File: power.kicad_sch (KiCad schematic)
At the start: 18 parts, among them U3 RT8096B

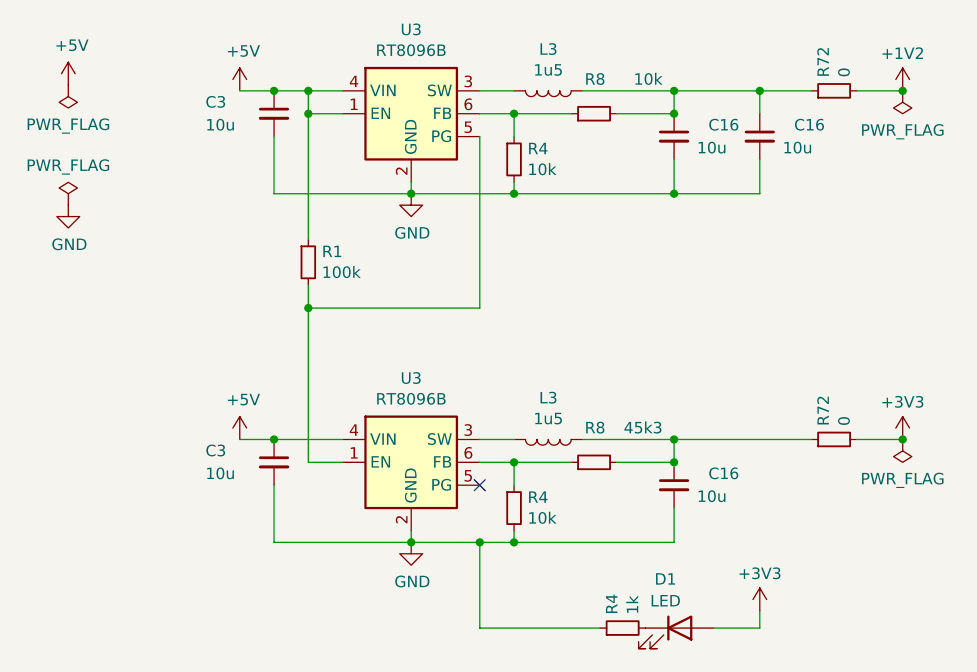
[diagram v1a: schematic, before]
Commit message: sdram layout done - COMPLETE REWORK NEEDED
cannot mix LVDS and GPIO banks due to too different timing
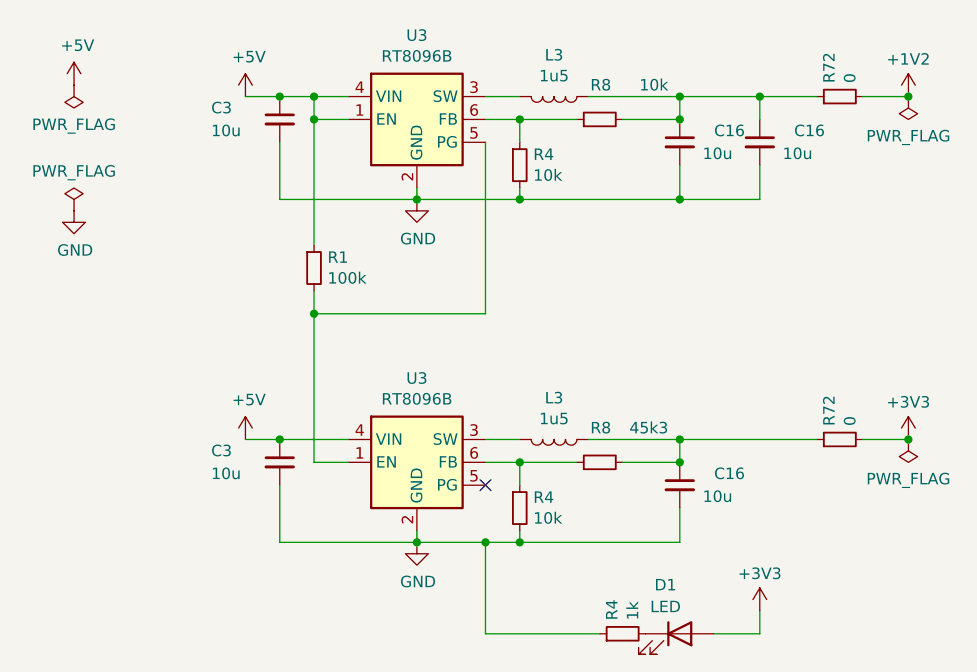
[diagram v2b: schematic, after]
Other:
- moved on the sheet: C16, C3, D1, L3, R1, R4, R72, R8, U3
